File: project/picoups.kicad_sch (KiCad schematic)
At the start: 42 parts, among them J1 Conn_02x20_Odd_Even, J2 BATT, J3 VIN, J4 5V, Q1 Q_PMOS_GSD, U1 LT3652EMSE, U2 INA3221, U3 TPS61235P

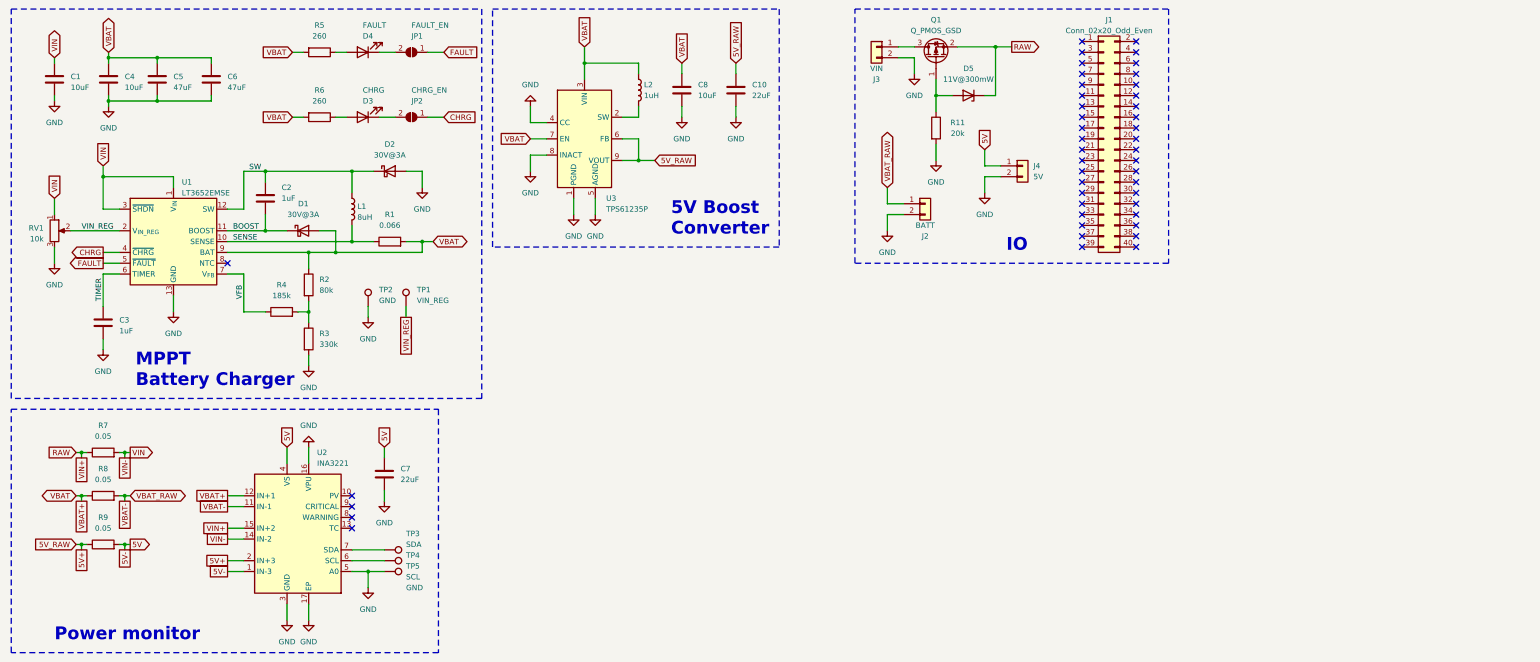
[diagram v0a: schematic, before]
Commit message: Revision 1 single page
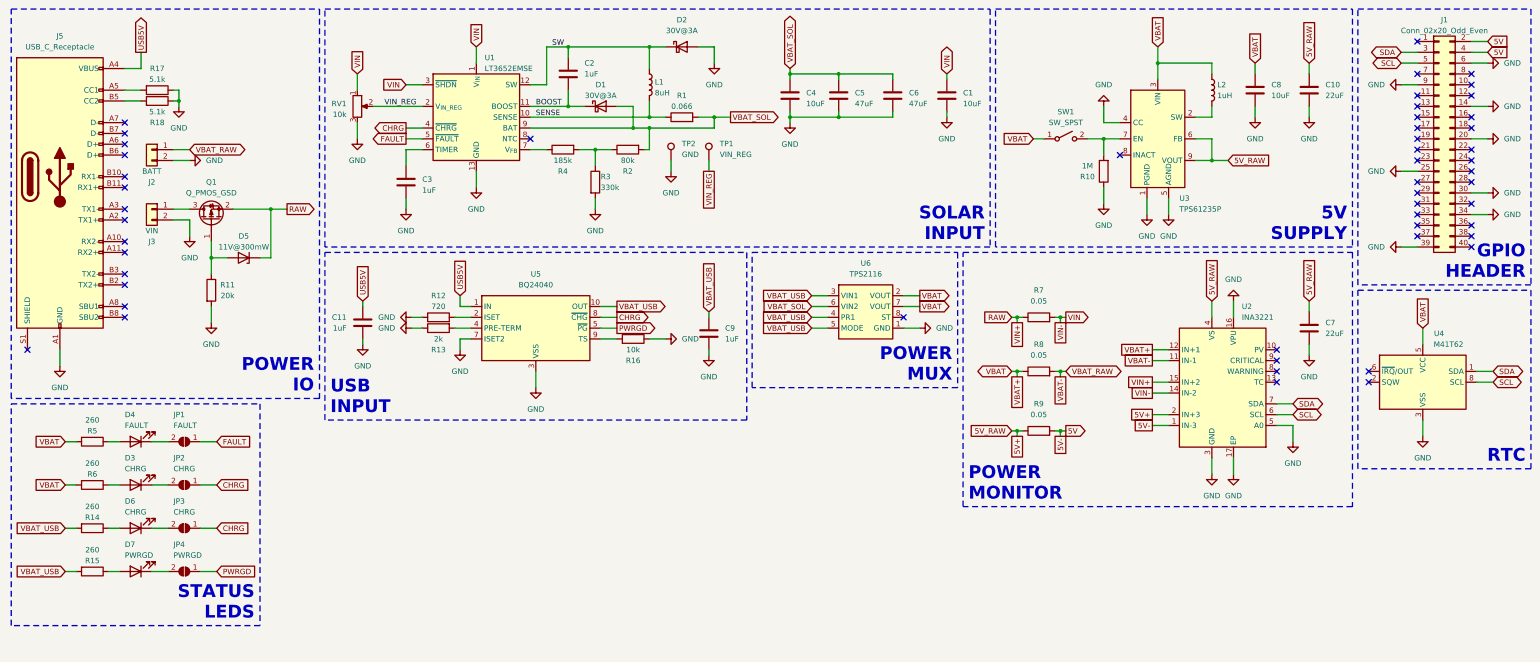
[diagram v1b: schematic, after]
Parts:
- removed J4: 5V, Connector_JST:JST_PH_S2B-PH-K_1x02_P2.00mm_Horizontal, symbol Connector_Generic:Conn_01x02
- removed TP3: SDA, TestPoint:TestPoint_Pad_D2.0mm, symbol Connector:TestPoint
- removed TP4: SCL, TestPoint:TestPoint_Pad_D2.0mm, symbol Connector:TestPoint
- removed TP5: GND, TestPoint:TestPoint_Pad_D2.0mm, symbol Connector:TestPoint
- added C11, C9: 1uF, Capacitor_SMD:C_0805_2012Metric, symbol Device:C
- added D6: CHRG, LED_SMD:LED_0805_2012Metric, symbol Device:LED
- added D7: PWRGD, LED_SMD:LED_0805_2012Metric, symbol Device:LED
- added J5: USB_C_Receptacle, symbol Connector:USB_C_Receptacle
- added JP3: CHRG, Jumper:SolderJumper-2_P1.3mm_Open_RoundedPad1.0x1.5mm, symbol Jumper:SolderJumper_2_Open
- added JP4: PWRGD, Jumper:SolderJumper-2_P1.3mm_Open_RoundedPad1.0x1.5mm, symbol Jumper:SolderJumper_2_Open
- added R10: 1M, Resistor_SMD:R_1210_3225Metric, symbol Device:R
- added R12: 720, Resistor_SMD:R_0805_2012Metric, symbol Device:R
- added R13: 2k, Resistor_SMD:R_0805_2012Metric, symbol Device:R
- added R14, R15: 260, Resistor_SMD:R_0805_2012Metric, symbol Device:R
- added R16: 10k, Resistor_SMD:R_0805_2012Metric, symbol Device:R
- added R17, R18: 5.1k, Resistor_SMD:R_0805_2012Metric, symbol Device:R
- added SW1: SW_SPST, symbol Switch:SW_SPST
- added U4: M41T62, symbol PicoUPS:M41T62
- added U5: BQ24040, symbol PicoUPS:BQ24040
- added U6: TPS2116, symbol PicoUPS:TPS2116
- JP1: value FAULT_EN -> FAULT
- JP2: value CHRG_EN -> CHRG
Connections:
- net 5V: now also J1.2 (Pin_2), J1.4 (Pin_4); no longer C7.1, U2.4 (VS)
- net 5V+: now also C7.1, U2.4 (VS)
- net CHRG: now also JP3.1 (A), U5.8 (~{CHG})
- net GND: now also J1.14 (Pin_14), J1.20 (Pin_20), J1.25 (Pin_25), J1.30 (Pin_30), J1.34 (Pin_34), J1.39 (Pin_39), J1.6 (Pin_6), J1.9 (Pin_9), C11.1, C9.2, J5.A1 (GND), J5.A12 (GND), J5.B1 (GND), J5.B12 (GND), R10.1, R12.1, R13.1, R16.1, R17.1, R18.1, U4.3 (VSS), U5.3 (VSS), U5.7 (ISET2), U6.1 (GND); no longer U3.8 (INACT)
- net VBAT: now also SW1.1 (A), U4.5 (VCC), U6.2 (VOUT), U6.7 (VOUT); no longer C4.1, C5.1, C6.1, D1.2 (A), R1.2, R2.1, U1.9 (BAT), U3.7 (EN)
- net SCL: now reaches U2.6 (SCL)
- net SCL: now also J1.5 (Pin_5), U4.8 (SCL)
- net SDA: now reaches U2.7 (SDA)
- net SDA: now also J1.3 (Pin_3), U4.1 (SDA)
- net at R3.1, R4.2: now also R2.1; no longer R2.2
- net TIMER: no longer names the net of C3.1, U1.6 (TIMER)
- net VFB: no longer names the net of R4.1, U1.7 (V_{FB})
- new net: D6.1 (K), JP3.2 (B)
- new net: D6.2 (A), R14.1
- new net: J5.B5 (CC2), R18.2
- new net: R10.2, SW1.2 (B), U3.7 (EN)
- new net: R13.2, U5.4 (PRE-TERM)
- new net: J5.A5 (CC1), R17.2
- new net: R12.2, U5.2 (ISET)
- new net: R16.2, U5.9 (TS)
- new net: D7.1 (K), JP4.2 (B)
- new net: D7.2 (A), R15.1
- new net PWRGD: JP4.1 (A), U5.5 (~{PG})
- new net USB5V: C11.2, J5.A4 (VBUS), J5.A9 (VBUS), J5.B4 (VBUS), J5.B9 (VBUS), U5.1 (IN)
- new net VBAT_SOL: C4.1, C5.1, C6.1, D1.2 (A), R1.2, R2.2, U1.9 (BAT), U6.6 (VIN2)
- new net VBAT_USB: C9.1, R14.2, R15.2, U5.10 (OUT), U6.3 (VIN1), U6.4 (PR1), U6.5 (MODE)
- no-connect marks 45 -> 52
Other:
- note added: "5V SUPPLY"
- note added: "GPIO HEADER"
- note added: "POWER IO"
- note added: "POWER MONITOR"
- note added: "POWER MUX"
- note added: "RTC"
- note added: "SOLAR INPUT"
- note added: "STATUS LEDS"
- note added: "USB INPUT"
- note removed: "5V Boost Converter"
- note removed: "IO"
- note removed: "MPPT Battery Charger"
- note removed: "Power monitor"
- title: (none) -> PicoUPS
- moved on the sheet: C1, C10, C2, C3, C4, C5, C6, C7, C8, D1, D2, D3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

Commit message: Revision 1 multi-page
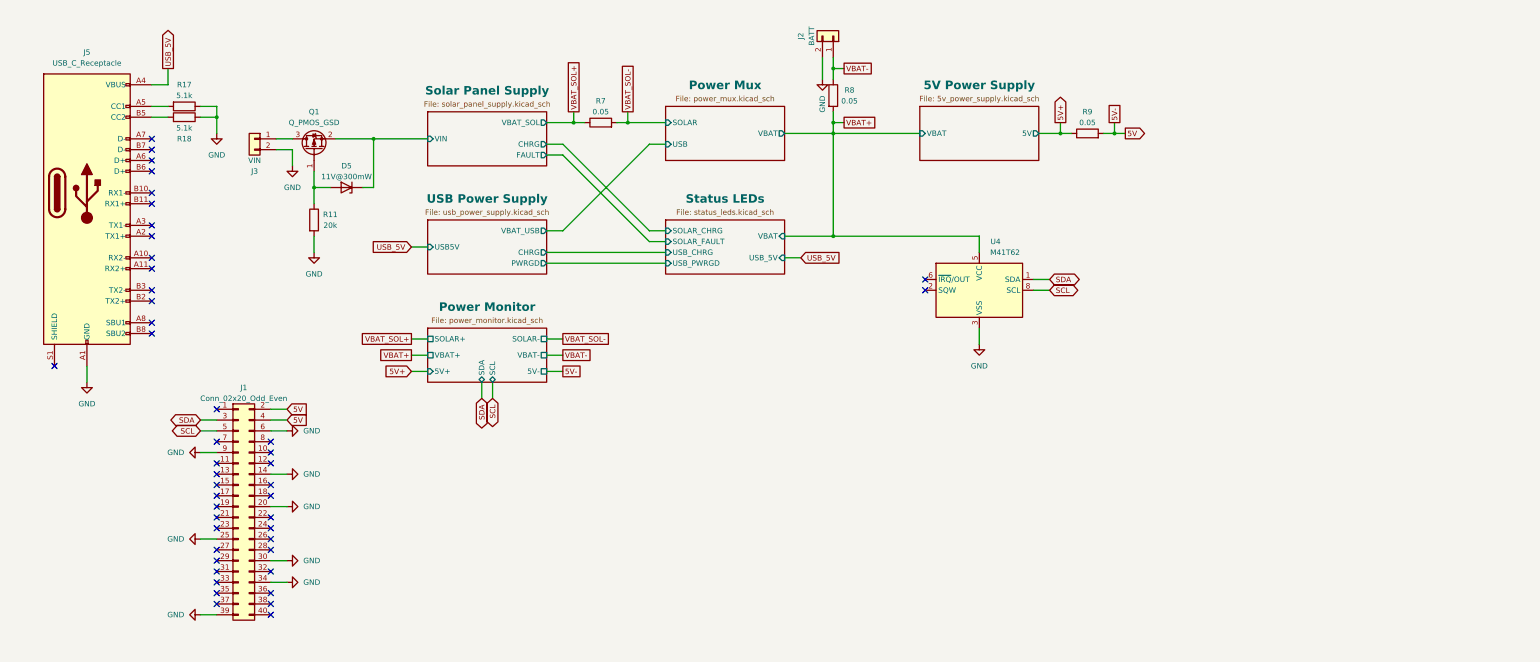
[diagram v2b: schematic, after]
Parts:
- removed C1, C4, C8: 10uF, Capacitor_SMD:C_0805_2012Metric, symbol Device:C
- removed C10, C7: 22uF, Capacitor_SMD:C_0805_2012Metric, symbol Device:C
- removed C11, C2, C3, C9: 1uF, Capacitor_SMD:C_0805_2012Metric, symbol Device:C
- removed C5, C6: 47uF, Capacitor_SMD:C_1210_3225Metric, symbol Device:C
- removed D1, D2: 30V@3A, Diode_SMD:D_SOD-123F, symbol Device:D_Schottky
- removed D3, D6: CHRG, LED_SMD:LED_0805_2012Metric, symbol Device:LED
- removed D4: FAULT, LED_SMD:LED_0805_2012Metric, symbol Device:LED
- removed D7: PWRGD, LED_SMD:LED_0805_2012Metric, symbol Device:LED
- removed JP1: FAULT, Jumper:SolderJumper-2_P1.3mm_Open_RoundedPad1.0x1.5mm, symbol Jumper:SolderJumper_2_Open
- removed JP2, JP3: CHRG, Jumper:SolderJumper-2_P1.3mm_Open_RoundedPad1.0x1.5mm, symbol Jumper:SolderJumper_2_Open
- removed JP4: PWRGD, Jumper:SolderJumper-2_P1.3mm_Open_RoundedPad1.0x1.5mm, symbol Jumper:SolderJumper_2_Open
- removed L1: 8uH, Inductor_SMD:L_Abracon_ASPI-4030S, symbol Device:L
- removed L2: 1uH, Inductor_SMD:L_Vishay_IHLP-2020, symbol Device:L
- removed R1: 0.066, Resistor_SMD:R_0805_2012Metric, symbol Device:R
- removed R10: 1M, Resistor_SMD:R_1210_3225Metric, symbol Device:R
- removed R12: 720, Resistor_SMD:R_0805_2012Metric, symbol Device:R
- removed R13: 2k, Resistor_SMD:R_0805_2012Metric, symbol Device:R
- removed R14, R15, R5, R6: 260, Resistor_SMD:R_0805_2012Metric, symbol Device:R
- removed R16: 10k, Resistor_SMD:R_0805_2012Metric, symbol Device:R
- removed R2: 80k, Resistor_SMD:R_0805_2012Metric, symbol Device:R
- removed R3: 330k, Resistor_SMD:R_0805_2012Metric, symbol Device:R
- removed R4: 185k, Resistor_SMD:R_0805_2012Metric, symbol Device:R
- removed RV1: 10k, PicoUPS:Potentiometer_Bourns_3214G_Horizontal, symbol Device:R_Potentiometer
- removed SW1: SW_SPST, symbol Switch:SW_SPST
- removed TP1: VIN_REG, TestPoint:TestPoint_Pad_D2.0mm, symbol Connector:TestPoint
- removed TP2: GND, TestPoint:TestPoint_Pad_D2.0mm, symbol Connector:TestPoint
- removed U1: LT3652EMSE, Package_SO:MSOP-12-1EP_3x4mm_P0.65mm_EP1.65x2.85mm, symbol Battery_Management:LT3652EMSE
- removed U2: INA3221, Package_DFN_QFN:Texas_RGV_S-PVQFN-N16_EP2.1x2.1mm, symbol Power_Management:INA3221
- removed U3: TPS61235P, PicoUPS:TPS61235P, symbol PicoUPS:TPS61235P
- removed U5: BQ24040, symbol PicoUPS:BQ24040
- removed U6: TPS2116, symbol PicoUPS:TPS2116
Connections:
- net VBAT-: now also R8.1; no longer R8.2
- net RAW renamed Solar Panel Supply/VIN
- net Solar Panel Supply/VIN: no longer R7.1
- net USB5V renamed USB_5V
- net VBAT renamed VBAT+
- net VBAT+: now also R8.2; no longer R8.1
- net VIN renamed VBAT_SOL-
- new net VBAT_SOL+: R7.1
- no-connect marks 52 -> 45
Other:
- added sheet 5V Power Supply (5v_power_supply.kicad_sch)
- added sheet Power Monitor (power_monitor.kicad_sch)
- added sheet Power Mux (power_mux.kicad_sch)
- added sheet Solar Panel Supply (solar_panel_supply.kicad_sch)
- added sheet Status LEDs (status_leds.kicad_sch)
- added sheet USB Power Supply (usb_power_supply.kicad_sch)
- note removed: "5V SUPPLY"
- note removed: "GPIO HEADER"
- note removed: "POWER IO"
- note removed: "POWER MONITOR"
- note removed: "POWER MUX"
- note removed: "RTC"
- note removed: "SOLAR INPUT"
- note removed: "STATUS LEDS"
- note removed: "USB INPUT"
- moved on the sheet: D5, J1, J3, J5, Q1, R11, R17, R18, U4
